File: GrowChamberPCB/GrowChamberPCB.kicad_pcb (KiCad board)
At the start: 2 copper layers, 190.3 x 105.6 mm, 154 parts, among them CN2 RelayBoard Interconnect, CN3 Connector_RB, J1 Mister, J10 FoggerBasin, J12 Moisture Sensor 3, J13 Moisture Sensor 2, J14 UART, J15 FAE Fan, J16 DrainLevel, J2 Moisture Sensor 1, J3 SCD30, J4 Heater Fans, J5 Fogger Solenoid, J6 Drain Solenoid, J7 Water Solenoid, J8 Glycol Solenoid, J9 CircFan, P1 12V_In, P2 12V_In, Q1 AO3400A_C347475, Q10 NPN, Q11 AO3400A_C347475, Q12 NPN, Q13 AO3400A_C347475, Q14 NPN, Q15 NPN, Q16 AO3400A_C347475, Q2 NPN, Q3 AO3400A_C347475, Q4 NPN, Q5 AO3400A_C347475, Q6 NPN, Q7 AO3400A_C347475, Q8 BRT30N70P3, Q9 NPN, SW1 Reset_Button_Internal, SW2 ResetButton_External, SW3 Bootmode_Internal, SW4 BootMode_External, U1 MP2393GTL-Z, U11 1N4007W, U12 1N4007W, U13 1N4007W, U14 1N4007W, U15 1N4007W, U16 1N4007W, U17 1N4007W, U19 To Faceplate, U2 MCP1826S-3302E/DB, U20 PCA9555APW,118, U3 ESP32-S3-WROOM-1U-N8R8, U4 To Faceplate, U5 1N4007W, U6 CR2013-MI2120, U7 TC4428EOA, U8 W25Q128JVSIQTR, U9 1N4007W

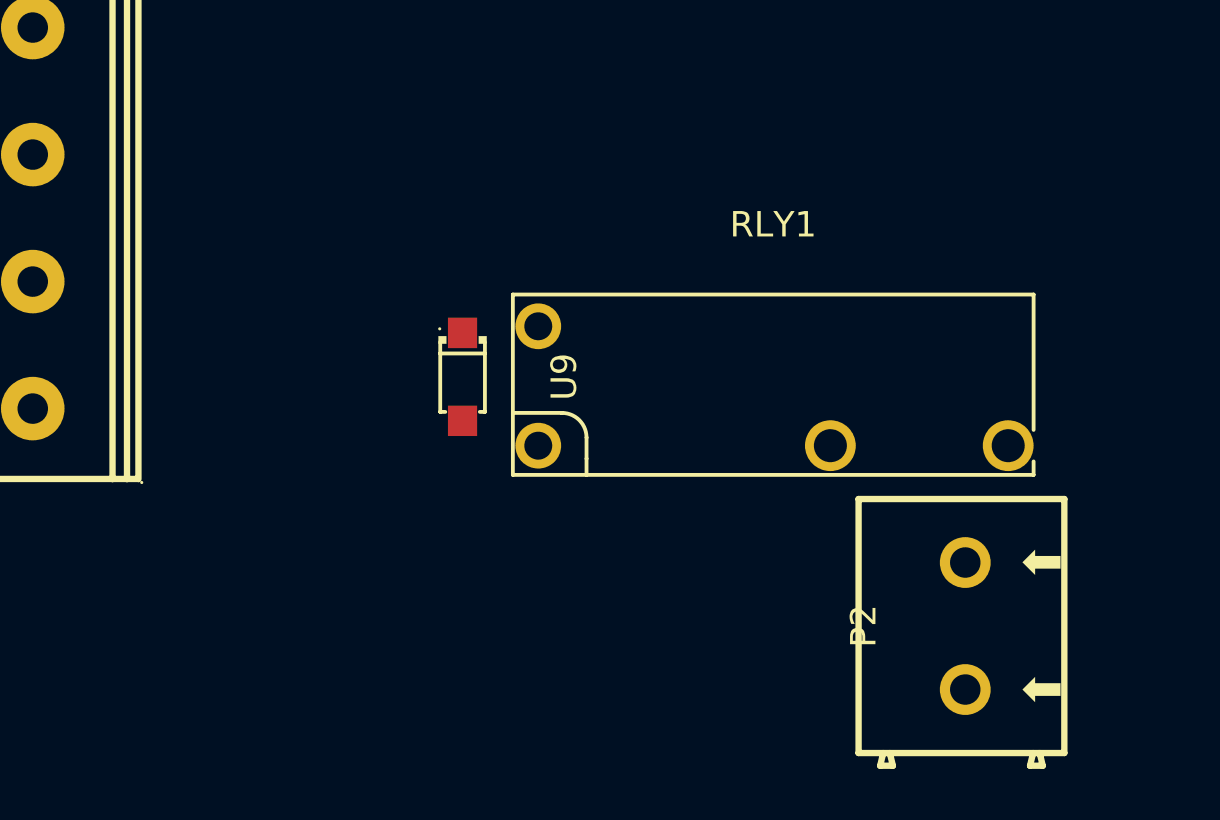
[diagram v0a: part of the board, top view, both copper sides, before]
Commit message: forgot to save pcb
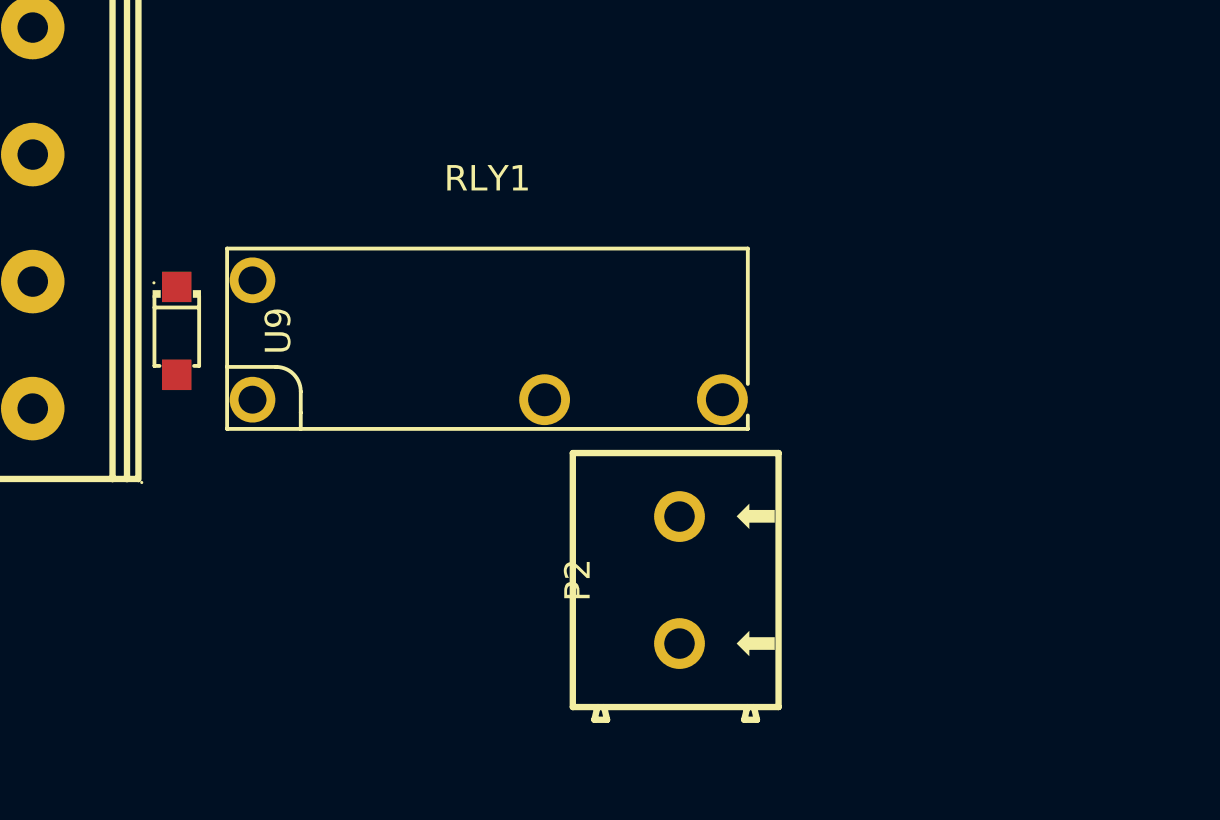
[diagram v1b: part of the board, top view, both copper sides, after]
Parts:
- moved RLY1 11.4 mm to (54.2, 171.4)
- moved U9 11.4 mm to (42.0, 171.1)
- moved P2 11.4 mm to (61.7, 180.9)
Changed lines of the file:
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@@
 	(footprint "easyeda2kicad:RELAY-TH_G5NB-1A-E-DCXX"
 		(layer "F.Cu")
-		(at 65.43 173.24)
+		(at 54.18 171.43)
 		(property "Reference" "RLY1"
 			(at 0 -6.35 0)
@@
 	(footprint "easyeda2kicad:SOD-123FL_L2.7-W1.8-LS3.7-RD"
 		(layer "F.Cu")
-		(at 53.2 172.88 -90)
+		(at 41.95 171.07 -90)
 		(property "Reference" "U9"
 			(at 0 -4 90)
@@
 	(footprint "easyeda2kicad:CONN-TH_2P-P5.00_CPC3703CTR"
 		(layer "F.Cu")
-		(at 72.99 182.69 90)
+		(at 61.74 180.88 90)
 		(descr "WJ127-5.0-2P")
 		(property "Reference" "P2"
